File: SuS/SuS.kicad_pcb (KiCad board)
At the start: 2 copper layers, 175.3 x 80.6 mm, 84 parts, among them P1 DIN41612_03x10_ABC, P2 DIN41612_03x10_ABC, Q1 BC556, U1 74HC245, U10 74HC32, U11 74HC245, U12 MAX691CPE, U13 74HC138, U14 74HC573, U15 74HC32, U16 74HC573, U17 74HC08, U18 74HC10, U19 74HC32, U2 27C4001, U20 74HC21, U21 MC68EC000FN, U22 RTC62421, U3 V62C5181024LL-70P, U4 74HC573, U6 27C4001, U7 V62C5181024LL-70P, U9 SG-531

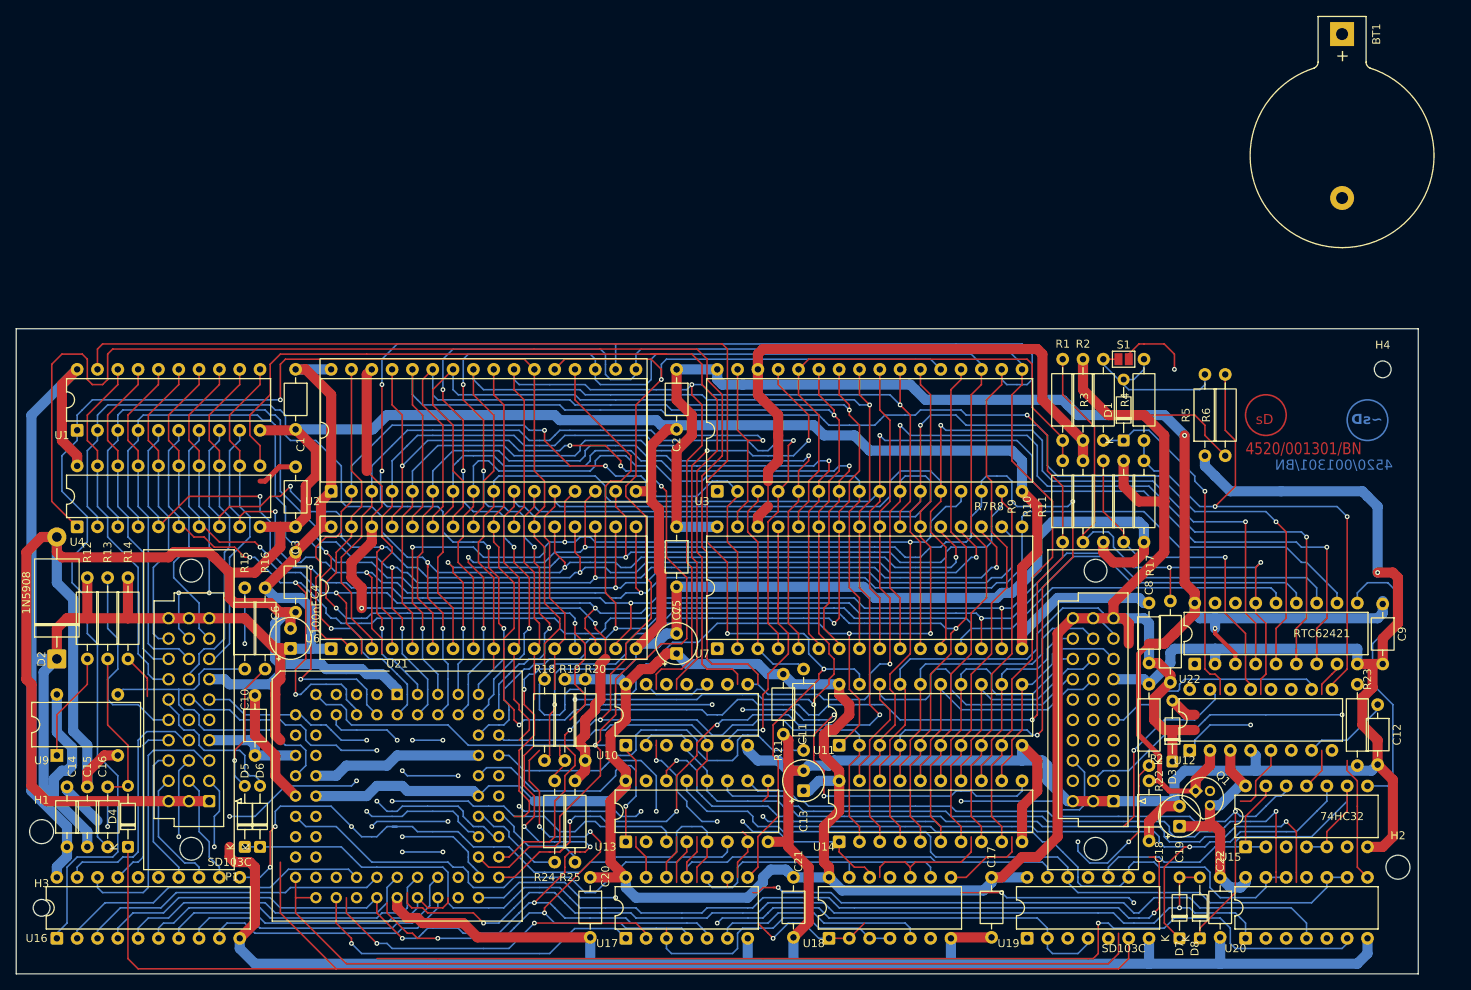
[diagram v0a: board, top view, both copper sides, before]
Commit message: alles verbunden
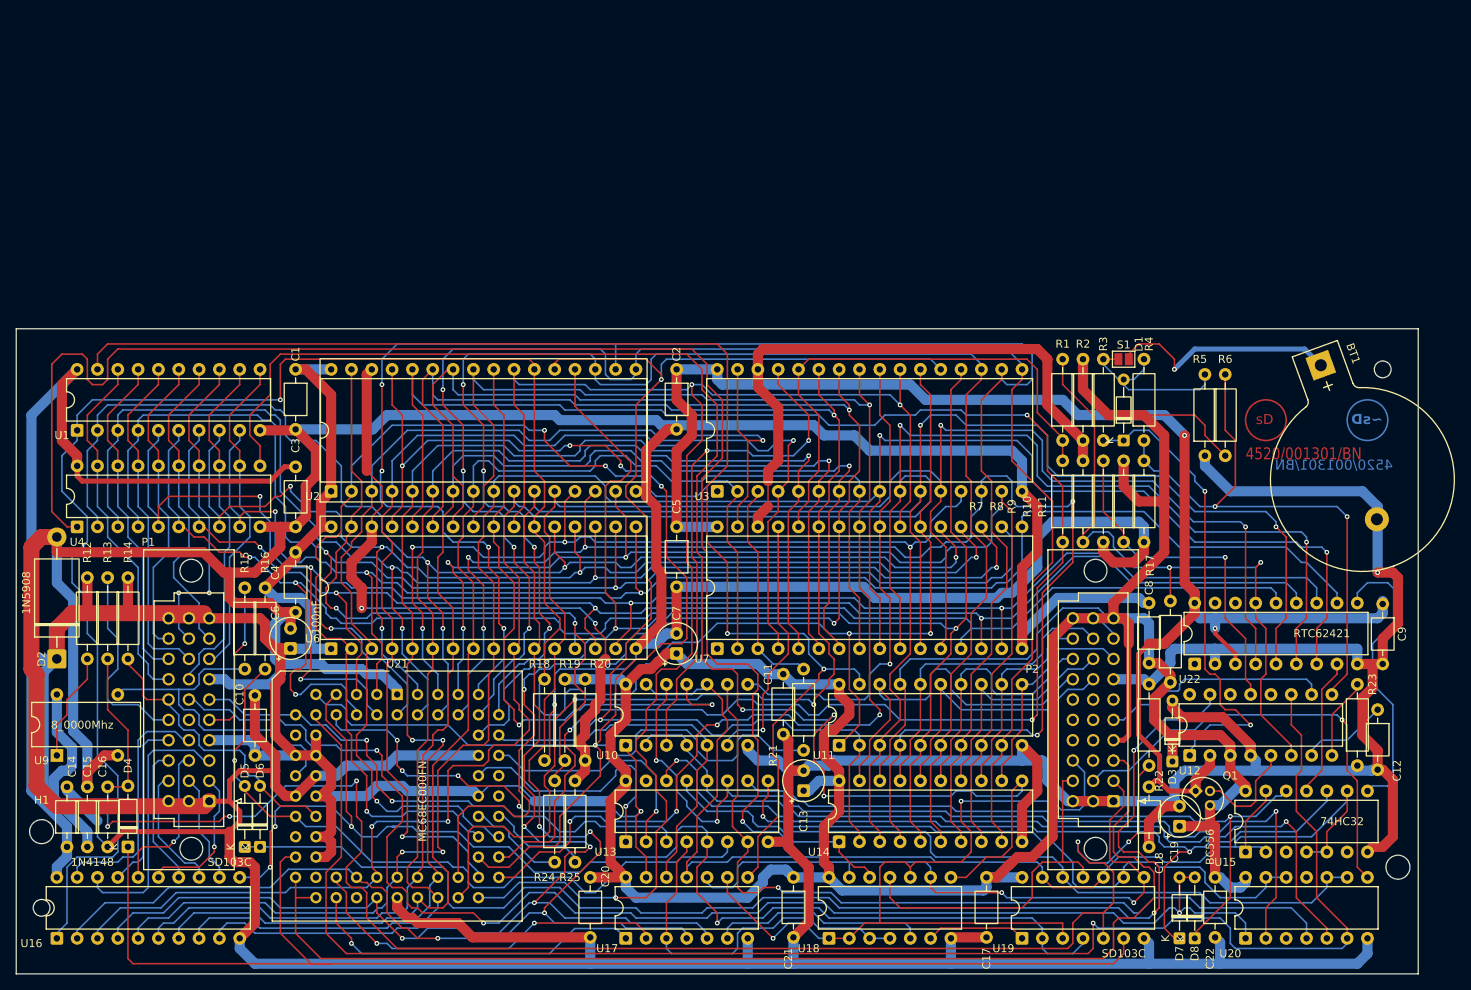
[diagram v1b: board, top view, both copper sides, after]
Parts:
- D4: value SD103C -> 1N4148; footprint Diode_THT:D_DO-34_SOD68_P7.62mm_Horizontal -> Diode_THT:D_DO-35_SOD27_P7.62mm_Horizontal
- U9: value SG-531 -> 8_0000Mhz
- moved BT1 41.5 mm to (217.7, 70.6), turned to -70 degrees
- moved C18 0.75 mm to (196.2, 130.8)
- moved C12 0.64 mm to (224.8, 113.7)
- moved C17 0.63 mm to (175.9, 134.6)
- moved C22 0.63 mm to (204.5, 134.6)
- moved D8 0.63 mm to (201.9, 142.2)
- moved U12 0.63 mm to (201.3, 119.4)
- moved U15 0.63 mm to (208.3, 131.4)
- moved U19 0.63 mm to (180.3, 142.2)
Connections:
- BT1 pad 1: unconnected-(BT1-+-Pad1) -> Net-(BT1-+)
- BT1 pad 2: unconnected-(BT1---Pad2) -> GND
- C10 pad 1: BR -> VCC
- C14 pad 2: Net-(C14-Pad2) -> GND
- C16 pad 1: Net-(C14-Pad2) -> GND
- C3 pad 1: unconnected-(C3-Pad1) -> VCC
- D4 pad 1: Net-(D4-K) -> BERR
- D5 pad 2: Net-(D5-A) -> HALT
- D6 pad 2: p1_c6 -> RESET
- D7 pad 2: Net-(D7-A) -> p1_b6
- D8 pad 1: Net-(D8-K) -> Y5
- D8 pad 2: Net-(D7-A) -> p1_b6
- P1 pad a2: unconnected-(P1A-Pin_a2-Pada2) -> EXT_A6
- P1 pad a4: BR -> VCC
- P1 pad a5: unconnected-(P1A-Pin_a5-Pada5) -> p1_a5
- P1 pad b3: unconnected-(P1B-Pin_b3-Padb3) -> EXT_A4
- P1 pad b5: p1_b5 -> unconnected-(P1B-Pin_b5-Padb5)
- P1 pad c6: p1_c6 -> RESET
- P2 pad a2: unconnected-(P2A-Pin_a2-Pada2) -> p2_a2
- P2 pad a3: unconnected-(P2A-Pin_a3-Pada3) -> IPL0
- P2 pad a4: unconnected-(P2A-Pin_a4-Pada4) -> VCC
- P2 pad b2: unconnected-(P2B-Pin_b2-Padb2) -> p2_b2
- P2 pad c2: unconnected-(P2C-Pin_c2-Padc2) -> p2_c2
- P2 pad c3: unconnected-(P2C-Pin_c3-Padc3) -> p2_c3
- Q1 pad 2: unconnected-(Q1-B-Pad2) -> Net-(Q1-B)
- R1 pad 2: Net-(U22-CS1) -> Net-(U12-~{LOW_LINE})
- R14 pad 1: unconnected-(R14-Pad1) -> RESET
- R15 pad 2: unconnected-(R15-Pad2) -> p1_a5
- R16 pad 1: Net-(D5-A) -> HALT
- R17 pad 2: Net-(U22-CS1) -> Net-(U12-~{LOW_LINE})
- R19 pad 1: Net-(R19-Pad1) -> Net-(U2-A18)
- R22 pad 1: Net-(R22-Pad1) -> Net-(D4-A)
- R23 pad 2: unconnected-(R23-Pad2) -> Net-(U12-OSC_SEL)
- R24 pad 2: Net-(R19-Pad1) -> Net-(U2-A18)
- R8 pad 1: Net-(U22-CS1) -> Net-(U12-~{LOW_LINE})
- S1 pad 2: unconnected-(S1-B-Pad2) -> Net-(BT1-+)
- U10 pad 1: unconnected-(U10-Pad1) -> UDS
- U10 pad 11: unconnected-(U10-Pad11) -> Net-(U2-~{OE})
- U10 pad 12: unconnected-(U10-Pad12) -> Y4
- U10 pad 3: unconnected-(U10-Pad3) -> Net-(U3-~{WE})
- U10 pad 9: unconnected-(U10-Pad9) -> Y7
- U12 pad 1: unconnected-(U12-VBATT-Pad1) -> Net-(D1-K)
- U12 pad 11: unconnected-(U12-WDI-Pad11) -> DTACK
- U12 pad 15: unconnected-(U12-~{RESET}-Pad15) -> Net-(D5-K)
- U12 pad 5: unconnected-(U12-BATT_ON-Pad5) -> Net-(Q1-B)
- U12 pad 6: unconnected-(U12-~{LOW_LINE}-Pad6) -> Net-(U12-~{LOW_LINE})
- U12 pad 8: unconnected-(U12-OSC_SEL-Pad8) -> Net-(U12-OSC_SEL)
- U13 pad 4: unconnected-(U13-~{E0}-Pad4) -> Net-(U13-~{E0})
- U13 pad 5: Net-(U13-~{E1}) -> AS
- U14 pad 11: unconnected-(U14-Load-Pad11) -> Net-(U14-Load)
- U15 pad 1: Net-(U15-Pad1) -> Net-(U10-Pad10)
- U15 pad 11: unconnected-(U15-Pad11) -> Net-(U22-~{RD})
- U15 pad 12: Net-(D8-K) -> Y5
- U15 pad 13: Net-(U15-Pad1) -> Net-(U10-Pad10)
- U15 pad 2: Net-(U15-Pad1) -> Net-(U10-Pad10)
- U15 pad 4: Net-(U15-Pad1) -> Net-(U10-Pad10)
- U15 pad 5: Net-(U15-Pad1) -> Net-(U10-Pad10)
- U15 pad 9: Net-(U15-Pad1) -> Net-(U10-Pad10)
- U16 pad 11: Net-(U13-~{E1}) -> AS
- U17 pad 10: Net-(U17-Pad10) -> p2_a2
- U17 pad 11: Net-(U17-Pad11) -> Net-(U10-Pad10)
- U17 pad 12: unconnected-(U17-Pad12) -> LDS
- U17 pad 13: unconnected-(U17-Pad13) -> UDS
- U17 pad 2: unconnected-(U17-Pad2) -> FC0
- U17 pad 3: Net-(U17-Pad3) -> Net-(U13-~{E0})
- U17 pad 4: unconnected-(U17-Pad4) -> A1
- U17 pad 9: unconnected-(U17-Pad9) -> p2_c3
- U18 pad 1: Net-(U18-Pad1) -> p2_c3
- U18 pad 10: unconnected-(U18-Pad10) -> p2_c3
- U18 pad 11: unconnected-(U18-Pad11) -> p2_c2
- U18 pad 13: Net-(U17-Pad10) -> p2_a2
- U18 pad 2: Net-(U18-Pad1) -> p2_c3
- U18 pad 3: Net-(U17-Pad3) -> Net-(U13-~{E0})
- U18 pad 4: Net-(U17-Pad3) -> Net-(U13-~{E0})
- U18 pad 6: unconnected-(U18-Pad6) -> Net-(U18-Pad6)
- U18 pad 8: unconnected-(U18-Pad8) -> Net-(U14-Load)
- U18 pad 9: Net-(U17-Pad10) -> p2_a2
- U19 pad 1: unconnected-(U19-Pad1) -> Net-(U18-Pad6)
- U19 pad 10: Net-(U15-Pad1) -> Net-(U10-Pad10)
- U19 pad 11: unconnected-(U19-Pad11) -> p2_c2
- U19 pad 13: Net-(U17-Pad11) -> Net-(U10-Pad10)
- U19 pad 2: Net-(U19-Pad2) -> AS
- U19 pad 3: unconnected-(U19-Pad3) -> p2_c3
- U19 pad 4: Net-(U19-Pad2) -> AS
- U19 pad 5: Net-(R22-Pad1) -> Net-(D4-A)
- U19 pad 6: Net-(D4-K) -> BERR
- U19 pad 8: Net-(U17-Pad10) -> p2_a2
- U19 pad 9: Net-(U19-Pad9) -> Y6
- U2 pad 31: A19 -> Net-(U2-A18)
- U20 pad 1: Net-(D7-A) -> p1_b6
- U20 pad 12: Net-(U19-Pad9) -> Y6
- U20 pad 13: Net-(U19-Pad9) -> Y6
- U20 pad 4: unconnected-(U20-Pad4) -> Y7
- U20 pad 6: unconnected-(U20-Pad6) -> DTACK
- U20 pad 8: unconnected-(U20-Pad8) -> p2_b2
- U21 pad 12: BG -> unconnected-(U21-~{BG}-Pad12)
- U21 pad 13: BGACK -> VCC
- U21 pad 14: BR -> VCC
- U21 pad 23: AVEC -> VCC
- U21 pad 25: IPL2 -> VCC
- U21 pad 28: FC2 -> unconnected-(U21-FC2-Pad28)
- U21 pad 31: A0 -> unconnected-(U21-A0-Pad31)
- U21 pad 52: A20 -> unconnected-(U21-A20-Pad52)
- U21 pad 54: A21 -> unconnected-(U21-A21-Pad54)
- U22 pad 15: Net-(U22-CS1) -> Net-(U12-~{LOW_LINE})
- U22 pad 8: unconnected-(U22-~{RD}-Pad8) -> Net-(U22-~{RD})
- U3 pad 29: unconnected-(U3-~{WE}-Pad29) -> Net-(U3-~{WE})
- U4 pad 1: unconnected-(U4-OE-Pad1) -> Net-(U14-OE)
- U4 pad 11: unconnected-(U4-Load-Pad11) -> Net-(U14-Load)
- U6 pad 31: A19 -> Net-(U2-A18)
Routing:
- net DTACK: track 0.00 -> 199.2 mm, vias 0 -> 1
- net Net-(U14-Load): track 0.00 -> 186.6 mm, vias 0 -> 3
- net Net-(U14-OE): track 19.9 -> 196.7 mm
- net Net-(D4-A): track 42.2 -> 210.1 mm, vias 3 -> 5
- net BERR: track 0.00 -> 160.1 mm
- net unconnected-(U4-OE-Pad1): track 159.3 -> 0.00 mm
- net Net-(D4-K): track 158.9 -> 0.00 mm
- net AS: track 0.00 -> 157.6 mm, vias 0 -> 4
- net Net-(U10-Pad10): track 8.67 -> 153.0 mm
- net p1_b6: track 26.9 -> 170.2 mm, vias 1 -> 3
- net unconnected-(U20-Pad6): track 129.7 -> 0.00 mm, vias 1 -> 0
- net Net-(D7-A): track 121.7 -> 0.00 mm, vias 2 -> 0
- net unconnected-(U4-Load-Pad11): track 117.0 -> 0.00 mm
- net p2_c3: track 0.00 -> 100.6 mm, vias 0 -> 2
- net Y7: track 6.50 -> 104.5 mm, vias 0 -> 1
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
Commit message: battok
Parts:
- S1: value Jumper_2_Open -> Batterie
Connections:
- net LDS renamed ~{LDS}
- net Net-(P2A-Pin_a5) renamed BATT_OK
- net Net-(U10-Pad10) renamed ~{DATA_VALID}
- net Net-(U13-~{E0}) renamed ~{SPACE_VALID}
- net UDS renamed ~{UDS}
